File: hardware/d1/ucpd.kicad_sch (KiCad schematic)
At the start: 48 parts, among them Q1 CSD17577Q3A, Q2 CSD17577Q3A, U15 ESDA25P35-1U1M, U16 ESDA25P35-1U1M, U3 TS3USB221RSER, U4 TCPP03-M20, U5 TCPP03-M20

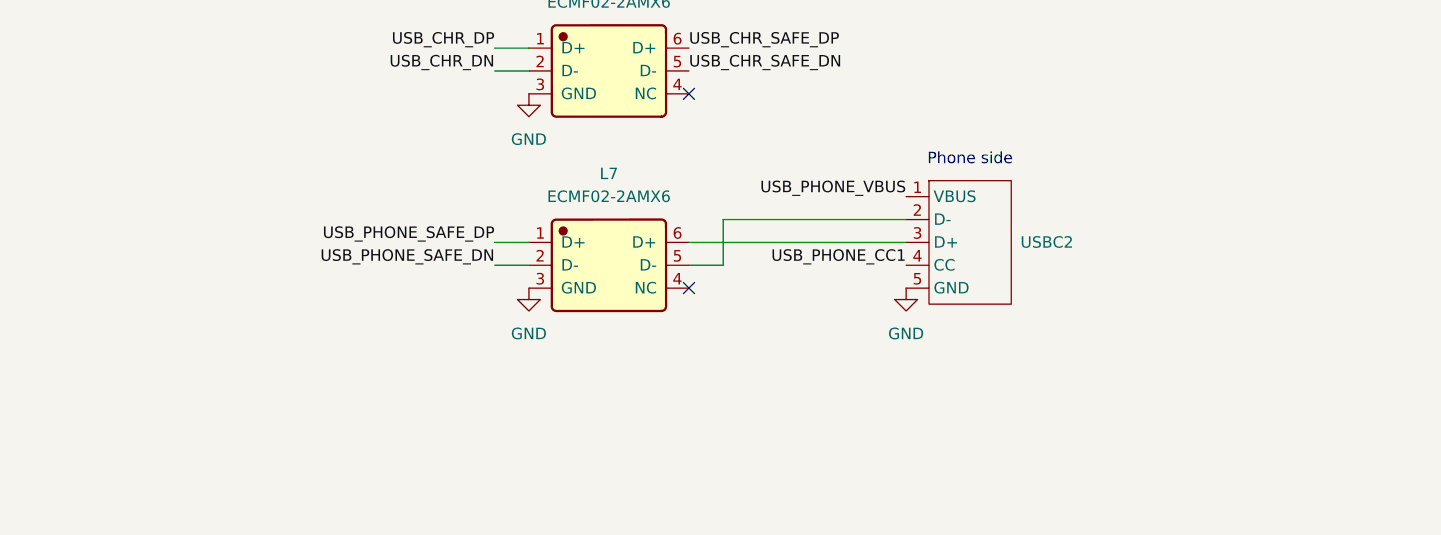
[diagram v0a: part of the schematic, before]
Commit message: Trace
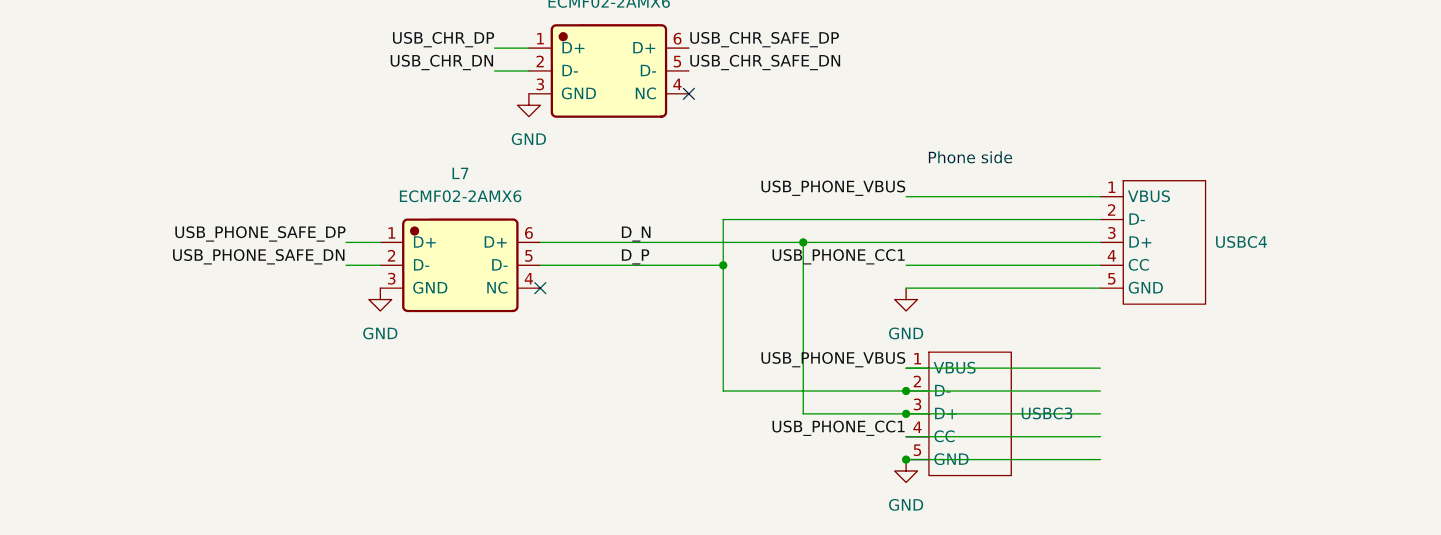
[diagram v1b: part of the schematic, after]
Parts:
- removed USBC2: (no value), JLCImport:USBC_EXT_5P, symbol JLCImport:USBC_5P_EXT
- added USBC3, USBC4: (no value), JLCImport:USBC_EXT_5P, symbol JLCImport:USBC_5P_EXT
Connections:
- net GND: now also USBC3.5 (GND), USBC4.5 (GND)
- net USB_PHONE_CC1: now also USBC3.4 (CC), USBC4.4 (CC)
- net USB_PHONE_VBUS: now also USBC3.1 (VBUS), USBC4.1 (VBUS)
- net D_P: now reaches L7.5 (D-)
- net D_P: now also USBC3.2 (D-), USBC4.2 (D-)
- net D_N: now reaches L7.6 (D+)
- net D_N: now also USBC3.3 (D+), USBC4.3 (D+)
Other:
- moved on the sheet: L7
